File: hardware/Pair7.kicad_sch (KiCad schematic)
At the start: 10 parts, among them IC7 TPS2HCS08AQPWPRQ1, J10 Conn_01x02, J18 Conn_01x02

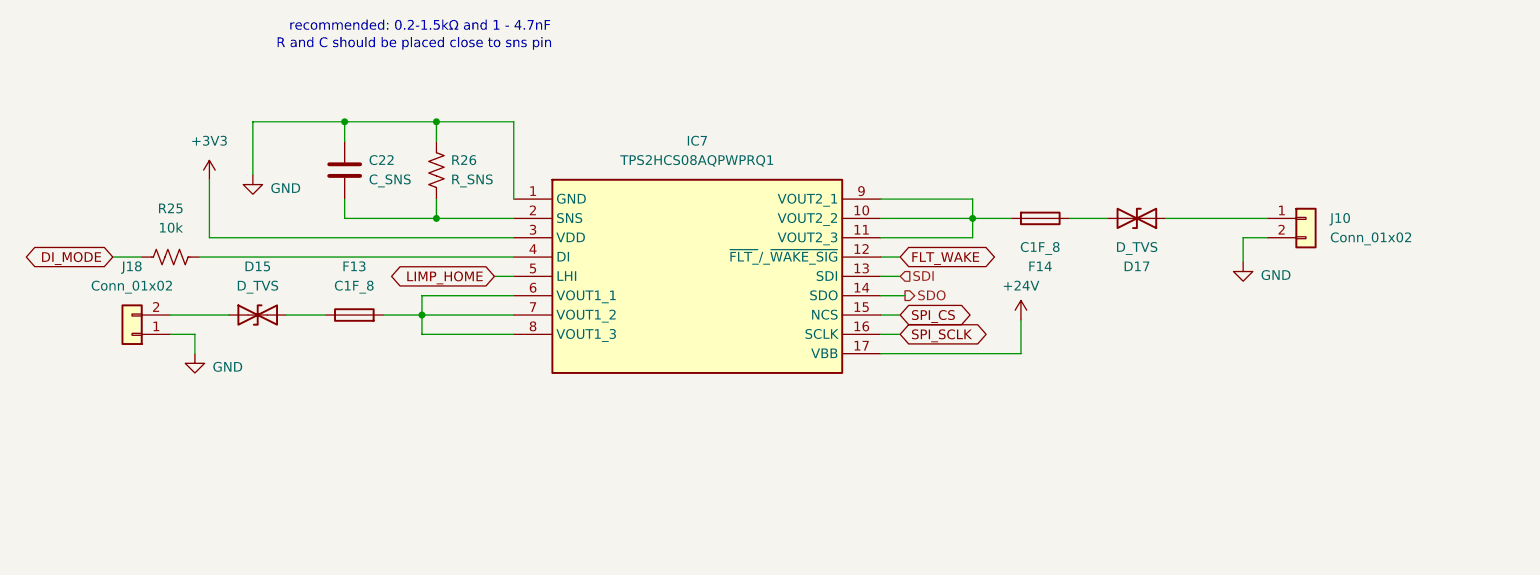
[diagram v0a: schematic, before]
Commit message: aesthetic added
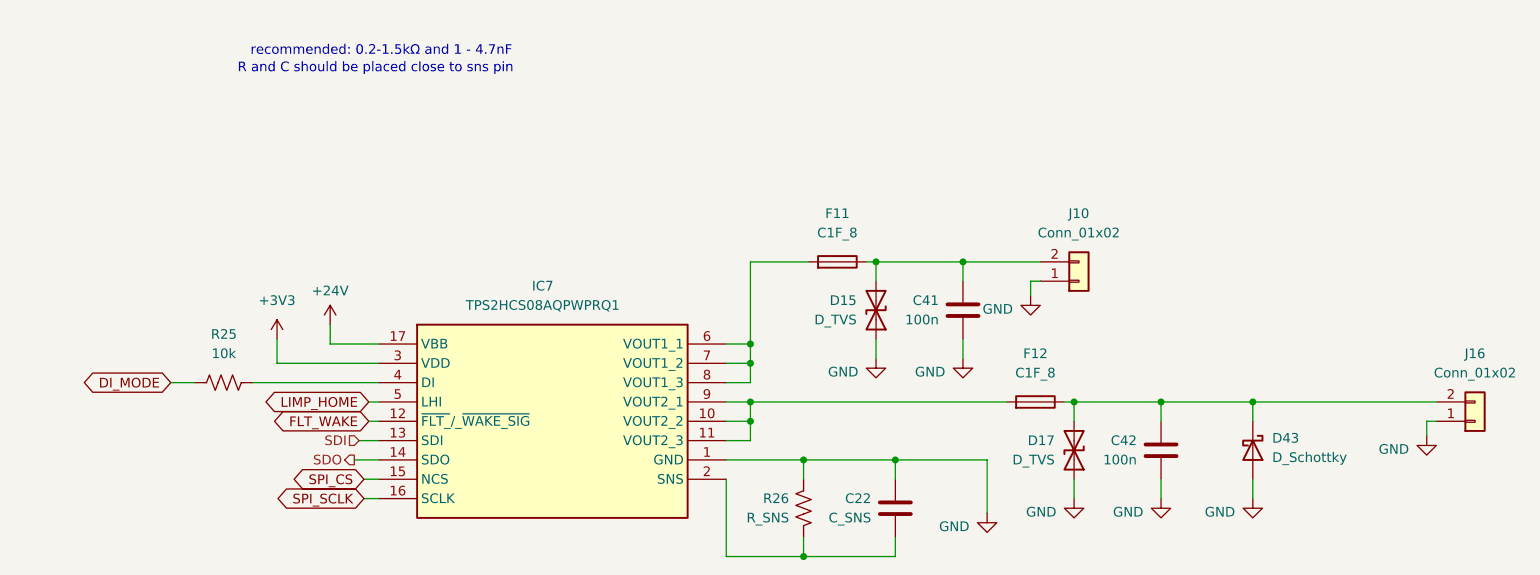
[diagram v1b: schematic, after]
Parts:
- removed F13, F14: C1F_8, Fuse:Fuse_1206_3216Metric, symbol PowerDistributionUnitLib:C1F_8
- removed J18: Conn_01x02, symbol Connector_Generic:Conn_01x02
- added C41, C42: 100n, symbol Device:C
- added D43: D_Schottky, symbol Device:D_Schottky
- added F11, F12: C1F_8, Fuse:Fuse_1206_3216Metric, symbol PowerDistributionUnitLib:C1F_8
- added J16: Conn_01x02, symbol Connector_Generic:Conn_01x02
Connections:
- net GND: now also D15.1 (A1), D17.1 (A1), J10.1 (Pin_1), C41.1, C42.1, D43.2 (A), J16.1 (Pin_1); no longer J10.2 (Pin_2)
- net at D17.2 (A2): now also C42.2, D43.1 (K), F12.1, J16.2 (Pin_2)
- net at IC7.10 (VOUT2_2), IC7.11 (VOUT2_3), IC7.9 (VOUT2_1): now also F12.2
- net at IC7.6 (VOUT1_1), IC7.7 (VOUT1_2), IC7.8 (VOUT1_3): now also F11.2
- net at D15.2 (A2): now also J10.2 (Pin_2), C41.2, F11.1
